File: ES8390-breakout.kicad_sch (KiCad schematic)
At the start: 64 parts, among them CN2 AV-5, CN3 Conn_01x14_Pin, CN4 PJ-327A, CN5 PJ-327A, CN6 AV-5, J1 Conn_01x02_Pin, J2 Conn_01x02_Pin, J3 AudioJack2, U1 LP5907MFX-3.0, U2 MAX98306xDT, U3 ES8390, U4 IM68A130AXTMA1, U6 TLV9062

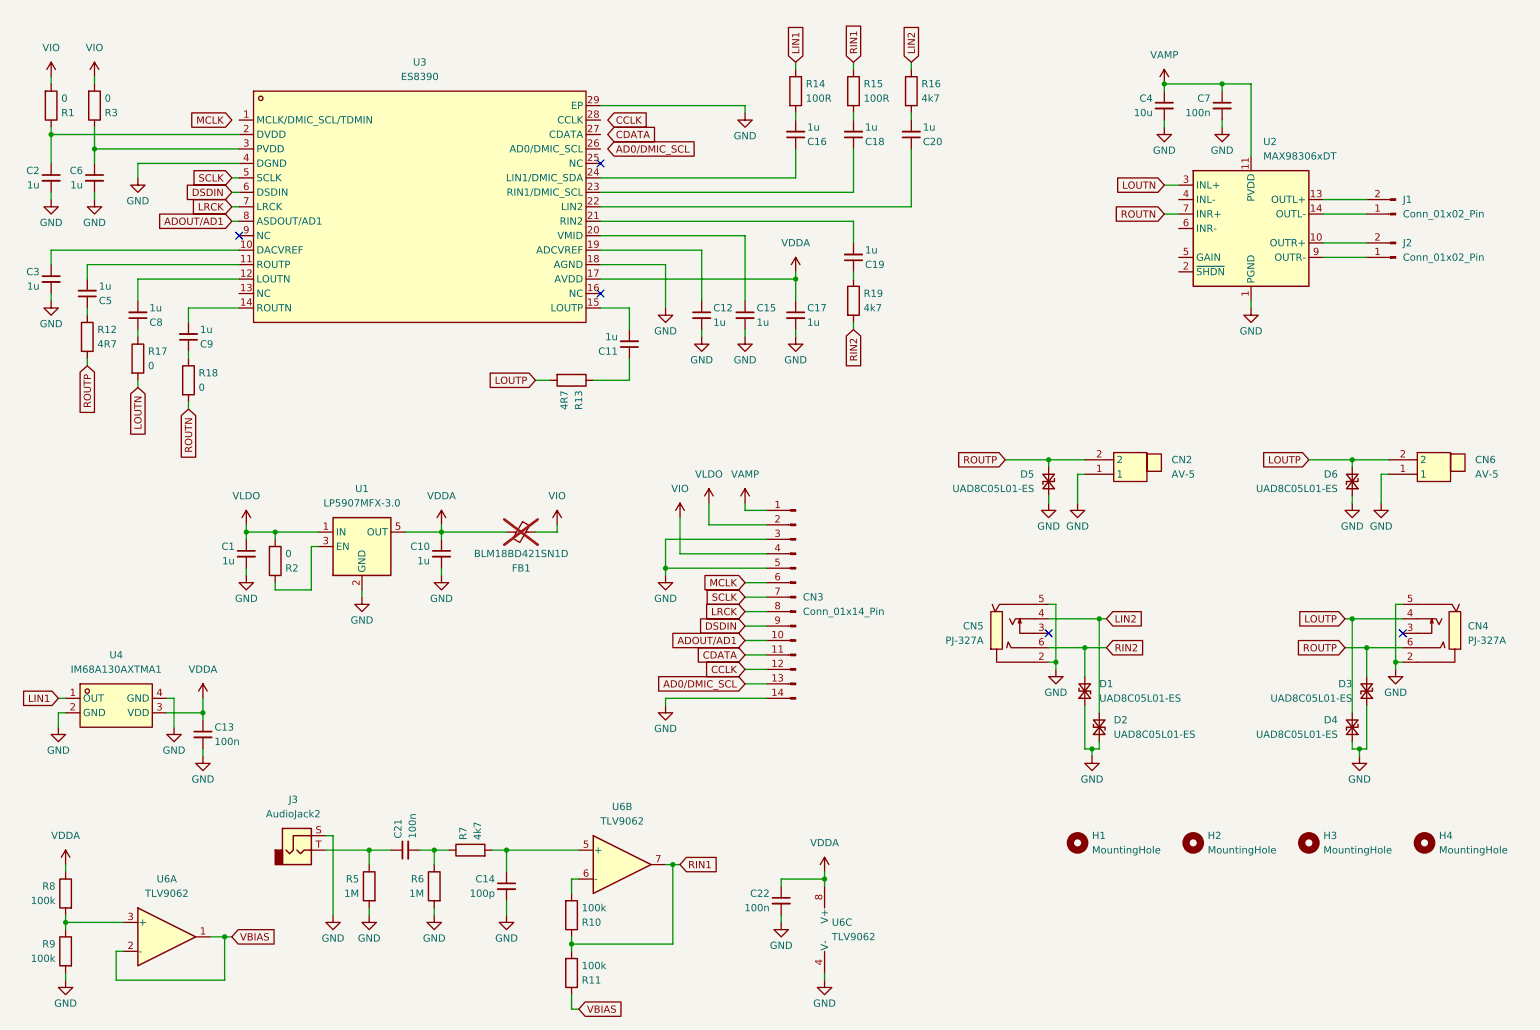
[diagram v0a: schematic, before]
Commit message: fix guitar input stage
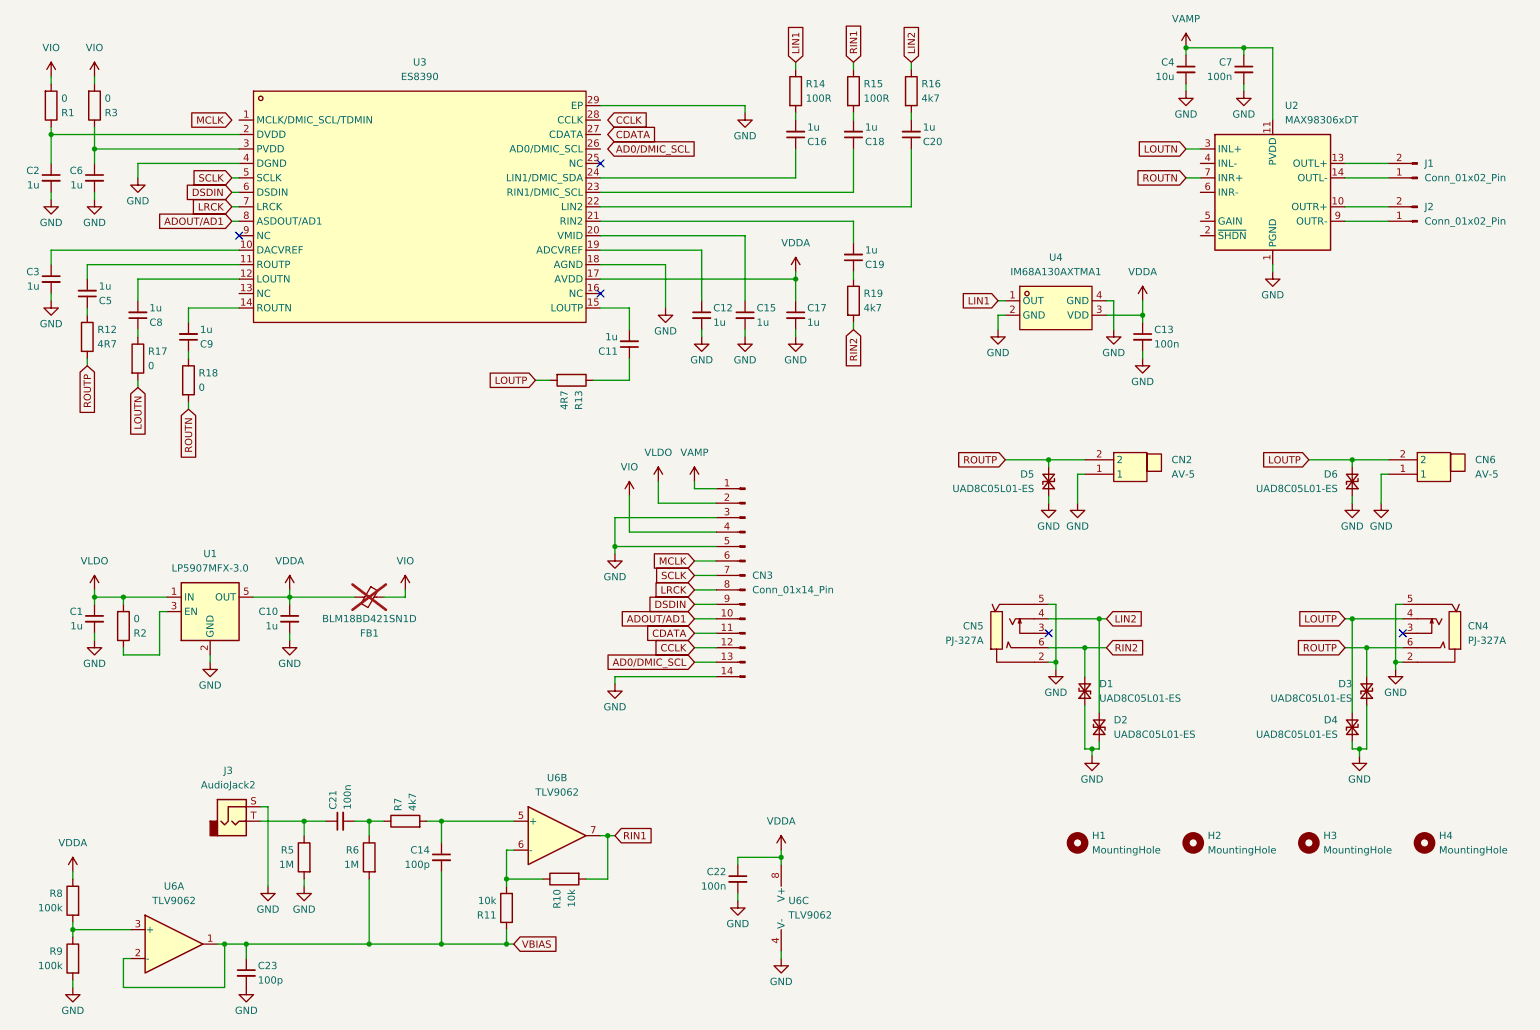
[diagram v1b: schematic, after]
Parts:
- added C23: 100p, Capacitor_SMD:C_0603_1608Metric, symbol Device:C_Small
- R10, R11: value 100k -> 10k
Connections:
- net GND: now also C23.2; no longer C14.2, R6.2
- net RIN1: now also R10.2; no longer R10.1, R11.2
- net VBIAS: now also C14.2, R6.2, C23.1
- net at U6.6 (-): now also R10.1, R11.2; no longer R10.2
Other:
- moved on the sheet: C1, C10, C13, C14, C21, C22, C4, C7, CN3, FB1, J1, J2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
